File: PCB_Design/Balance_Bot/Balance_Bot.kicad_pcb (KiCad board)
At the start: 2 copper layers, 22 parts, among them J1 LEFT_MOTOR, J2 RIGHT_MOTOR, J3 12V_BAT, J4 Conn_01x08_Socket, U1 MPU-6050, U2 DRV8871DDA, U4 DRV8871DDA

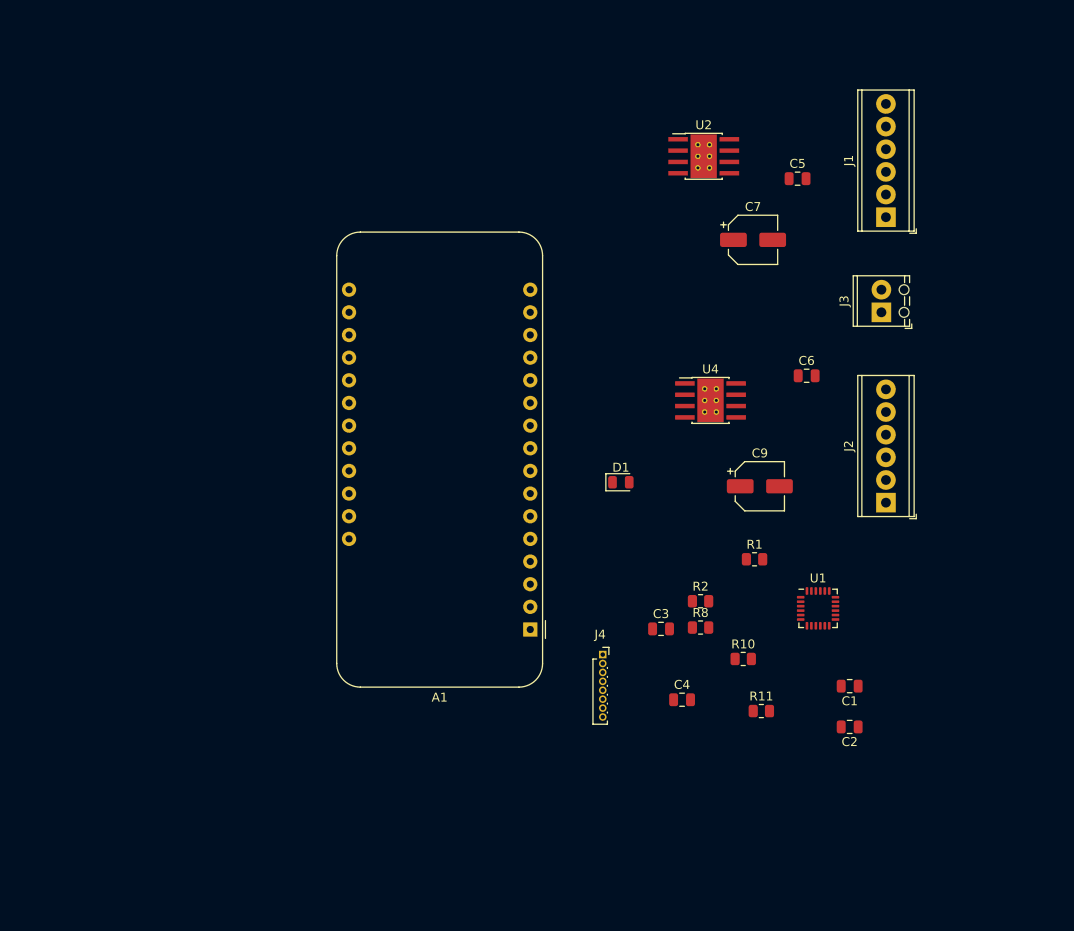
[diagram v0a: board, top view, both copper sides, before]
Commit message: board design
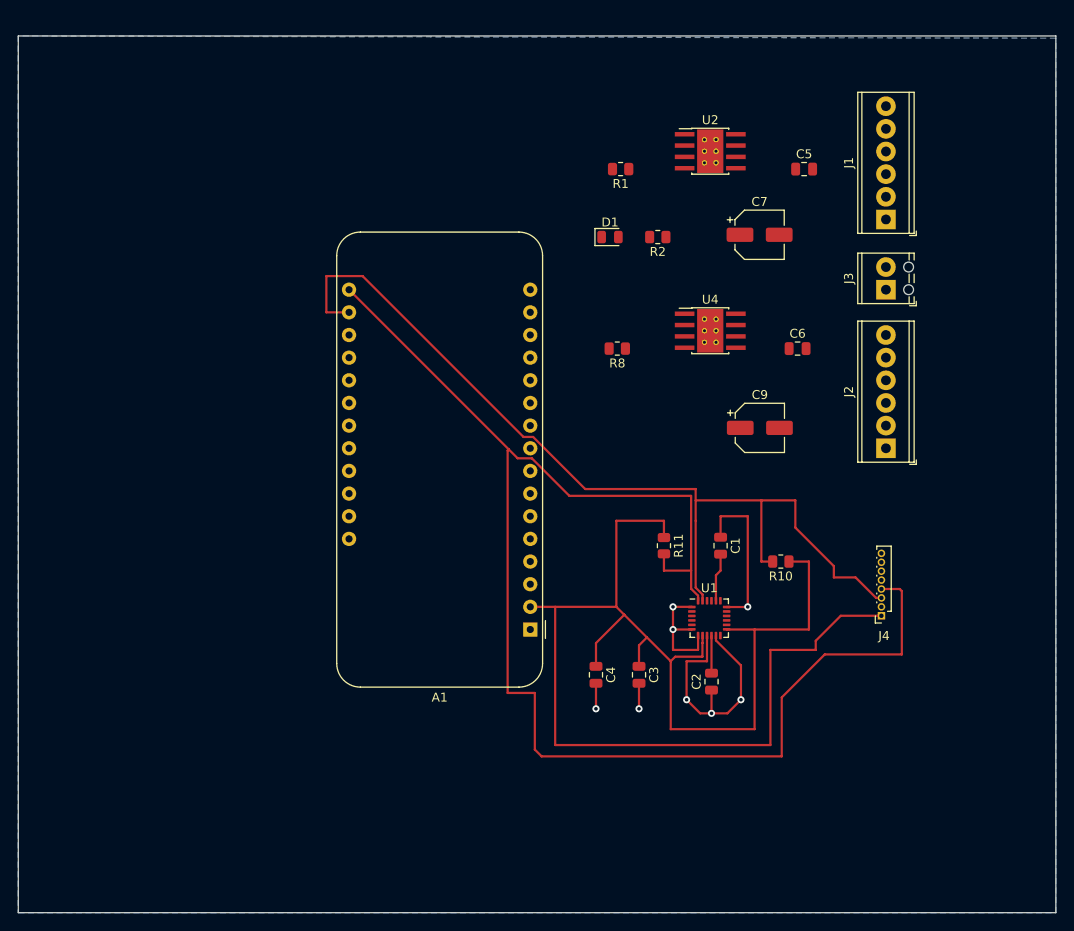
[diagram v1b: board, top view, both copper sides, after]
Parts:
- moved R1 46.3 mm to (160.8, 77.7), turned to 180 degrees
- moved R2 41.1 mm to (164.9, 85.3), turned to 180 degrees
- moved R8 32.6 mm to (160.4, 97.8), turned to 180 degrees
- moved J4 31.5 mm to (190.0, 127.7), turned to 180 degrees
- moved D1 27.5 mm to (159.6, 85.3)
- moved R11 21.5 mm to (165.6, 119.9), turned to -90 degrees
- moved C1 21.4 mm to (172.0, 119.9), turned to -90 degrees
- moved C2 16.3 mm to (170.9, 135.1), turned to 90 degrees
- moved U1 12.3 mm to (170.7, 128.0)
- moved R10 11.7 mm to (178.7, 121.7), turned to 180 degrees
- moved C4 10.0 mm to (158.0, 134.4), turned to -90 degrees
- moved U4 7.81 mm to (170.8, 95.8)
- moved C9 6.54 mm to (176.4, 106.7)
- moved J2 6.10 mm to (190.5, 109.0)
- moved C3 5.71 mm to (162.8, 134.4), turned to -90 degrees
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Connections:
- J4 pad 1: +3V3 -> +3.3V
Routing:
- net +3.3V: track 0.00 -> 164.2 mm
- net SDA: track 0.00 -> 161.3 mm
- net SCL: track 0.00 -> 106.8 mm
- net GND: track 0.00 -> 64.9 mm, vias 0 -> 8
- net Net-(U1-CPOUT): track 0.00 -> 5.44 mm
- net Net-(U1-REGOUT): track 0.00 -> 4.21 mm
- added copper zone on B.Cu, net GND
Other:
- board outline added: 116.3 x 98.3 mm

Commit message: board
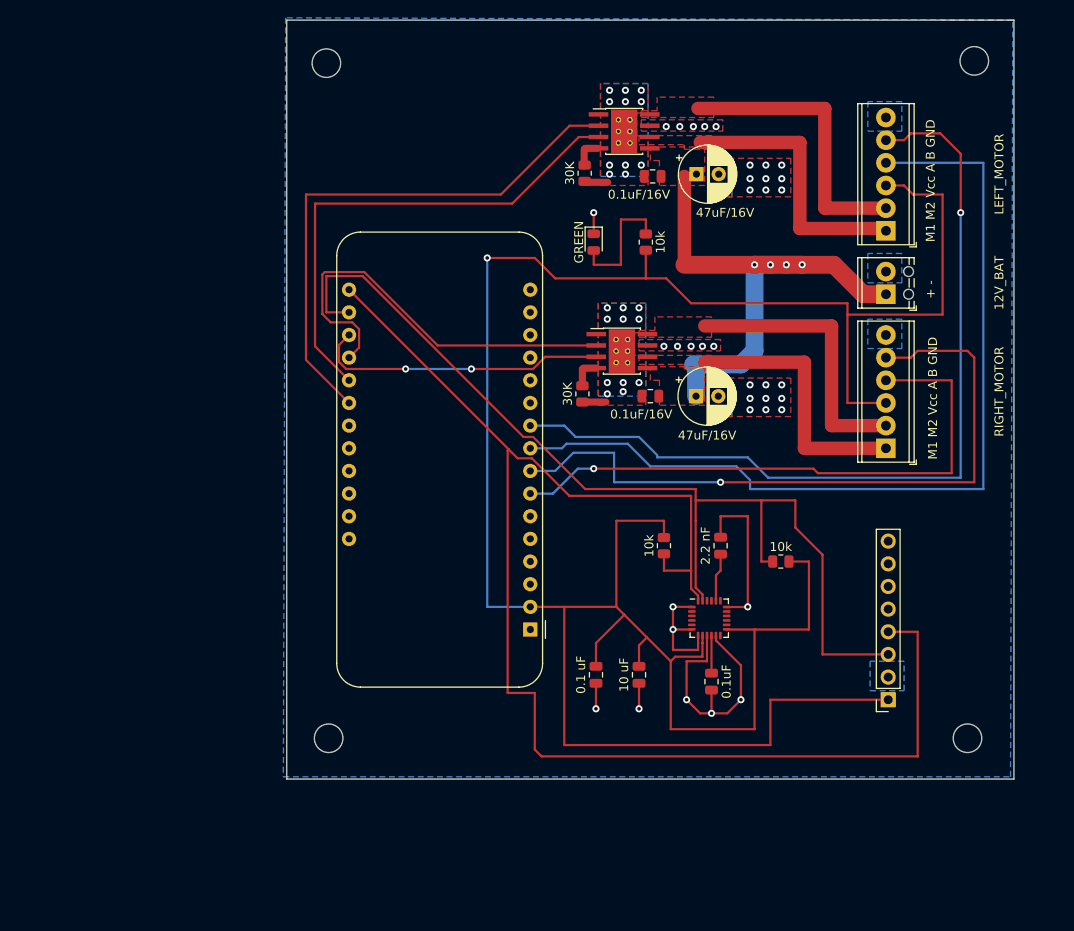
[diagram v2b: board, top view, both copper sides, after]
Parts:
- added H1: MountingHole, MountingHole:MountingHole_3.2mm_M3, F.Cu at (127.8, 65.8)
- added H2: MountingHole, MountingHole:MountingHole_3.2mm_M3, F.Cu at (200.4, 65.5)
- added H3: MountingHole, MountingHole:MountingHole_3.2mm_M3, F.Cu at (199.6, 141.5)
- added H4: MountingHole, MountingHole:MountingHole_3.2mm_M3, F.Cu at (128.0, 141.5)
- C5, C6: value 0.1uF/12V -> 0.1uF/16V
- C7, C9: value 47uF/12V -> 47uF/16V; footprint Capacitor_SMD:CP_Elec_5x5.3 -> Capacitor_THT:CP_Radial_D6.3mm_P2.50mm
- J4: footprint Connector_PinSocket_1.00mm:PinSocket_1x08_P1.00mm_Vertical -> Connector_PinSocket_2.54mm:PinSocket_1x08_P2.54mm_Vertical
- moved C6 17.4 mm to (164.1, 103.1), turned to 180 degrees
- moved C5 17.0 mm to (164.3, 78.5), turned to 180 degrees
- moved U4 10.2 mm to (160.9, 98.1)
- moved U2 9.91 mm to (161.1, 73.4)
- moved C7 9.82 mm to (169.3, 78.2)
- moved J4 9.44 mm to (190.8, 137.2)
- moved C9 7.99 mm to (169.2, 103.1)
- moved R8 6.41 mm to (156.5, 102.9), turned to -90 degrees
- moved R1 4.06 mm to (156.7, 78.1), turned to -90 degrees
- moved D1 1.91 mm to (157.7, 85.9), turned to -90 degrees
- moved R2 1.46 mm to (163.6, 85.9), turned to 90 degrees
- moved J1 1.27 mm to (190.5, 84.6)
- moved J3 0.51 mm to (190.5, 91.7)
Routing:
- net +3.3V: track 164.2 -> 292.1 mm, vias 0 -> 1
- net OUT_A_LEFT: track 0.00 -> 101.2 mm
- net OUT_B_LEFT: track 0.00 -> 97.0 mm, vias 0 -> 1
- net OUT_B_RIGHT: track 0.00 -> 78.4 mm, vias 0 -> 1
- net OUT_A_RIGHT: track 0.00 -> 66.4 mm, vias 0 -> 1
- net IN2_LEFT: track 0.00 -> 61.4 mm
- net 12V_BAT: track 0.00 -> 60.0 mm, vias 0 -> 4
- net IN1_LEFT: track 0.00 -> 56.3 mm
- net IN2_RIGHT: track 0.00 -> 47.1 mm
- net IN1_RIGHT: track 0.00 -> 33.2 mm, vias 0 -> 2
- net Net-(J2-Pin_2): track 0.00 -> 31.5 mm
- net Net-(J1-Pin_2): track 0.00 -> 31.5 mm
- net Net-(J2-Pin_1): track 0.00 -> 30.0 mm
- net Net-(J1-Pin_1): track 0.00 -> 30.0 mm
- net Net-(D1-A): track 0.00 -> 14.2 mm
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- added copper zone on F.Cu, net 12V_BAT
- added copper zone on F.Cu, net GND
- added copper zone on F.Cu, net Net-(J1-Pin_1)
- added copper zone on F.Cu, net Net-(J1-Pin_2)
- added copper zone on F.Cu, net Net-(J2-Pin_1)
- added copper zone on F.Cu, net Net-(J2-Pin_2)
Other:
- board size 116.3 x 98.3 mm -> 81.5 x 85.1 mm
- board text added: "+ -"
- board text added: "M1 M2 Vcc A B GND"
